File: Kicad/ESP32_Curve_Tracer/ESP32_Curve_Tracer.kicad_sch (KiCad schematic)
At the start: 69 parts, among them J1 PROBE_CH1-, J2 PROBE_CH2-, J3 PROBE_CH1_VIA1_16, J4 PROBE_CH2_VIA1_16, J5 PROBE_CH1+, J6 PROBE_CH2+, U1 DOIT-ESP32-DEVKIT-V1, U2 LMV324, U3 CD74HC4067M, U4 CD74HC4067M, U5 CD74HC4067M, U6 CD74HC4067M, U7 74HC595, U8 74HC595, U9 74HC595

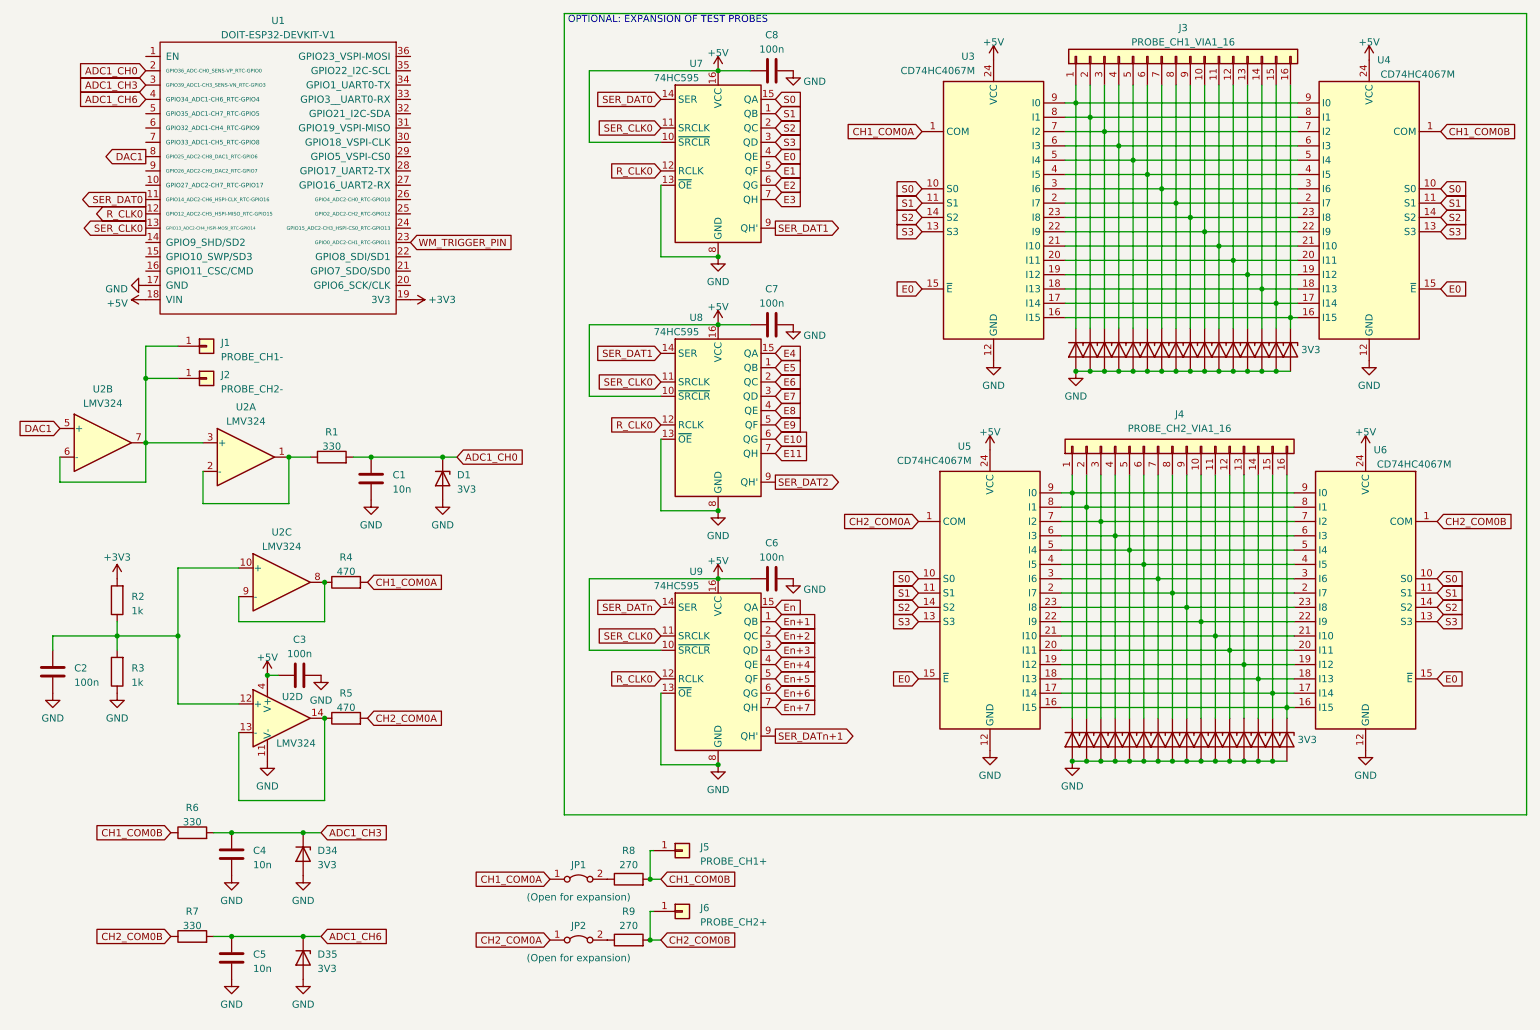
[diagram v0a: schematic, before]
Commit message: Update
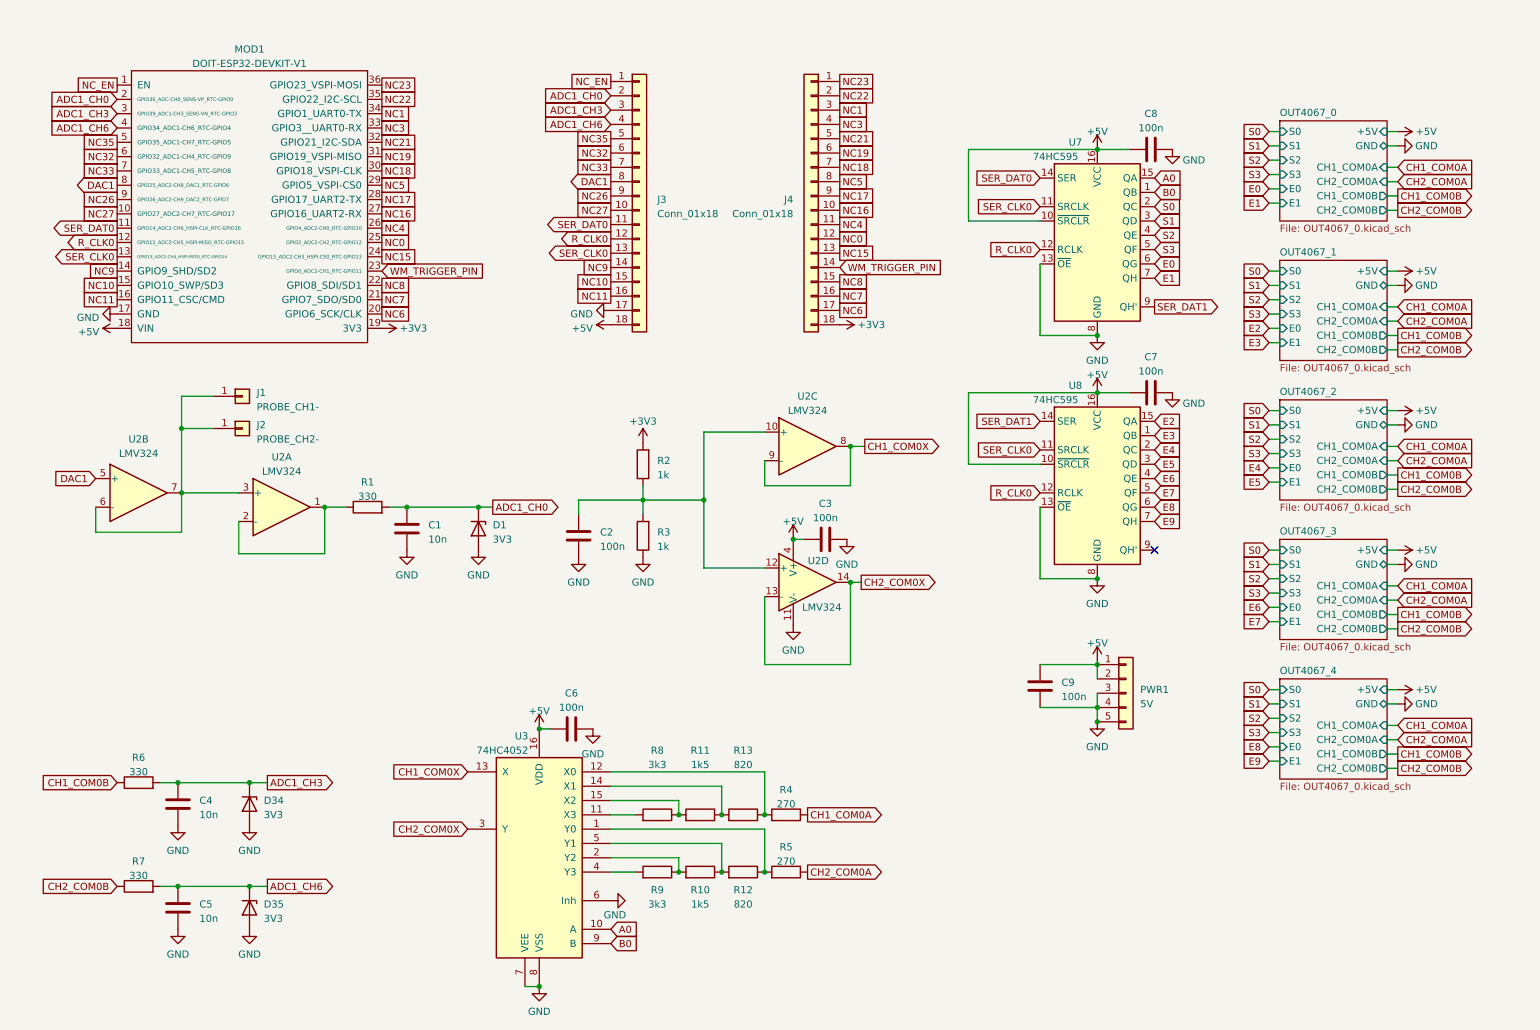
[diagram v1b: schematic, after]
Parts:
- removed D10, D11, D12, D13, D14, D15, D16, D17, D18, D19, D2, D20, D21, D22, D23, D24, D25, D26, D27, D28, D29, D3, D30, D31, D32, D33, D4, D5, D6, D7, D8, D9: 3V3, symbol Device:D_Zener
- removed J3: PROBE_CH1_VIA1_16, symbol Connector_Generic:Conn_01x16
- removed J4: PROBE_CH2_VIA1_16, symbol Connector_Generic:Conn_01x16
- removed J5: PROBE_CH1+, symbol Connector_Generic:Conn_01x01
- removed J6: PROBE_CH2+, symbol Connector_Generic:Conn_01x01
- removed JP1, JP2: (Open for expansion), symbol Jumper:Jumper_2_Bridged
- removed U3, U4, U5, U6: CD74HC4067M, Package_SO:SOIC-24W_7.5x15.4mm_P1.27mm, symbol 74xx:CD74HC4067M
- removed U9: 74HC595, symbol 74xx:74HC595
- added C9: 100n, Capacitor_SMD:C_0805_2012Metric_Pad1.18x1.45mm_HandSolder, symbol Device:C
- added J3, J4: Conn_01x18, Connector_PinSocket_2.54mm:PinSocket_1x18_P2.54mm_Vertical, symbol Connector_Generic:Conn_01x18
- added PWR1: 5V, Connector_PinHeader_2.54mm:PinHeader_1x05_P2.54mm_Vertical, symbol Connector_Generic:Conn_01x05
- added R10, R11: 1k5, Resistor_SMD:R_0805_2012Metric_Pad1.20x1.40mm_HandSolder, symbol Device:R
- added R12, R13: 820, Resistor_SMD:R_0805_2012Metric_Pad1.20x1.40mm_HandSolder, symbol Device:R
- added U3: 74HC4052, Package_SO:SOP-16_3.9x9.9mm_P1.27mm, symbol 4xxx:4052
- C1, C2, C3, C4, C5, C6, C7, C8: footprint (none) -> Capacitor_SMD:C_0805_2012Metric_Pad1.18x1.45mm_HandSolder
- D1, D34, D35: footprint (none) -> Diode_SMD:D_SOD-323_HandSoldering
- J1, J2: footprint (none) -> Connector_PinHeader_2.54mm:PinHeader_1x01_P2.54mm_Vertical
- MOD1: renamed from U1; footprint (none) -> ESP32:ESP32-DOIT-DEVKIT
- R1, R2, R3, R6, R7: footprint (none) -> Resistor_SMD:R_0805_2012Metric_Pad1.20x1.40mm_HandSolder
- R4, R5: value 470 -> 270; footprint (none) -> Resistor_SMD:R_0805_2012Metric_Pad1.20x1.40mm_HandSolder
- R8, R9: value 270 -> 3k3; footprint (none) -> Resistor_SMD:R_0805_2012Metric_Pad1.20x1.40mm_HandSolder
- U2: footprint (none) -> Package_SO:SO-14_3.9x8.65mm_P1.27mm
- U7, U8: footprint (none) -> Package_SO:SOP-16_3.9x9.9mm_P1.27mm
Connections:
- net E10 is gone; now on net E8: U8.6 (QG)
- net E11 is gone; now on net E9: U8.7 (QH)
- net +3V3: now also J4.18 (Pin_18)
- net +5V: now also C9.1, J3.18 (Pin_18), PWR1.1 (Pin_1), PWR1.2 (Pin_2), U3.16 (VDD)
- net ADC1_CH0: now also J3.2 (Pin_2)
- net ADC1_CH3: now also J3.3 (Pin_3)
- net ADC1_CH6: now also J3.4 (Pin_4)
- net CH1_COM0A: now also R4.1; no longer R4.2
- net CH1_COM0B: no longer R8.2
- net CH2_COM0A: now also R5.1; no longer R5.2
- net CH2_COM0B: no longer R9.2
- net DAC1: now also J3.8 (Pin_8)
- net E0: now also U7.6 (QG); no longer U7.4 (QE)
- net E1: now also U7.7 (QH); no longer U7.5 (QF)
- net E2: now also U8.15 (QA); no longer U7.6 (QG)
- net E3: now also U8.1 (QB); no longer U7.7 (QH)
- net E4: now also U8.2 (QC); no longer U8.15 (QA)
- net E5: now also U8.3 (QD); no longer U8.1 (QB)
- net E6: now also U8.4 (QE); no longer U8.2 (QC)
- net E7: now also U8.5 (QF); no longer U8.3 (QD)
- net E8: no longer U8.4 (QE)
- net E9: no longer U8.5 (QF)
- net GND: now also C9.2, J3.17 (Pin_17), PWR1.3 (Pin_3), PWR1.4 (Pin_4), PWR1.5 (Pin_5), U3.6 (Inh), U3.7 (VEE), U3.8 (VSS)
- net R_CLK0: now also J3.12 (Pin_12)
- net S0: now also U7.2 (QC); no longer U7.15 (QA)
- net S1: now also U7.3 (QD); no longer U7.1 (QB)
- net S2: now also U7.4 (QE); no longer U7.2 (QC)
- net S3: now also U7.5 (QF); no longer U7.3 (QD)
- net SER_CLK0: now also J3.13 (Pin_13)
- net SER_DAT0: now also J3.11 (Pin_11)
- net WM_TRIGGER_PIN: now also J4.14 (Pin_14)
- net at R9.1: now also R10.2, U3.2 (Y2)
- net at R8.1: now also R11.2, U3.15 (X2)
- net CH2_COM0X: now reaches U2.13 (-), U2.14
- net CH2_COM0X: now also U3.3 (Y); no longer R5.1
- net NC_EN: now reaches MOD1.1 (EN)
- net NC_EN: now also J3.1 (Pin_1)
- net NC27: now reaches MOD1.10 (GPIO27_ADC2-CH7_RTC-GPIO17)
- net NC27: now also J3.10 (Pin_10)
- net NC9: now reaches MOD1.14 (GPIO9_SHD/SD2)
- net NC9: now also J3.14 (Pin_14)
- net NC10: now reaches MOD1.15 (GPIO10_SWP/SD3)
- net NC10: now also J3.15 (Pin_15)
- net NC11: now reaches MOD1.16 (GPIO11_CSC/CMD)
- net NC11: now also J3.16 (Pin_16)
- net NC6: now reaches MOD1.20 (GPIO6_SCK/CLK)
- net NC6: now also J4.17 (Pin_17)
- net NC7: now reaches MOD1.21 (GPIO7_SDO/SD0)
- net NC7: now also J4.16 (Pin_16)
- net NC8: now reaches MOD1.22 (GPIO8_SDI/SD1)
- net NC8: now also J4.15 (Pin_15)
- net NC15: now reaches MOD1.24 (GPIO15_ADC2-CH3_HSPI-CS0_RTC-GPIO13)
- net NC15: now also J4.13 (Pin_13)
- net NC0: now reaches MOD1.25 (GPIO2_ADC2-CH2_RTC-GPIO12)
- net NC0: now also J4.12 (Pin_12)
- net NC4: now reaches MOD1.26 (GPIO4_ADC2-CH0_RTC-GPIO10)
- net NC4: now also J4.11 (Pin_11)
- net NC16: now reaches MOD1.27 (GPIO16_UART2-RX)
- net NC16: now also J4.10 (Pin_10)
- net NC17: now reaches MOD1.28 (GPIO17_UART2-TX)
- net NC17: now also J4.9 (Pin_9)
- net NC5: now reaches MOD1.29 (GPIO5_VSPI-CS0)
- net NC5: now also J4.8 (Pin_8)
- net NC18: now reaches MOD1.30 (GPIO18_VSPI-CLK)
- net NC18: now also J4.7 (Pin_7)
- net NC19: now reaches MOD1.31 (GPIO19_VSPI-MISO)
- net NC19: now also J4.6 (Pin_6)
- net NC21: now reaches MOD1.32 (GPIO21_I2C-SDA)
- net NC21: now also J4.5 (Pin_5)
- net NC3: now reaches MOD1.33 (GPIO3__UART0-RX)
- net NC3: now also J4.4 (Pin_4)
- net NC1: now reaches MOD1.34 (GPIO1_UART0-TX)
- net NC1: now also J4.3 (Pin_3)
- net NC22: now reaches MOD1.35 (GPIO22_I2C-SCL)
- net NC22: now also J4.2 (Pin_2)
- net NC23: now reaches MOD1.36 (GPIO23_VSPI-MOSI)
- net NC23: now also J4.1 (Pin_1)
- net NC35: now reaches MOD1.5 (GPIO35_ADC1-CH7_RTC-GPIO5)
- net NC35: now also J3.5 (Pin_5)
- net NC32: now reaches MOD1.6 (GPIO32_ADC1-CH4_RTC-GPIO9)
- net NC32: now also J3.6 (Pin_6)
- net NC33: now reaches MOD1.7 (GPIO33_ADC1-CH5_RTC-GPIO8)
- net NC33: now also J3.7 (Pin_7)
- net NC26: now reaches MOD1.9 (GPIO26_ADC2-CH9_DAC2_RTC-GPIO7)
- net NC26: now also J3.9 (Pin_9)
- net CH1_COM0X: now reaches U2.8, U2.9 (-)
- net CH1_COM0X: now also U3.13 (X); no longer R4.1
- net SER_DAT2: no longer names the net of U8.9 (QH')
- new net: R11.1, R13.2, U3.14 (X1)
- new net: R13.1, R4.2, U3.12 (X0)
- new net: R12.1, R5.2, U3.1 (Y0)
- new net: R10.1, R12.2, U3.5 (Y1)
- new net: R9.2, U3.4 (Y3)
- new net: R8.2, U3.11 (X3)
- new net A0: U3.10 (A), U7.15 (QA)
- new net B0: U3.9 (B), U7.1 (QB)
- no-connect marks 0 -> 1
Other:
- added sheet OUT4067_0 (OUT4067_0.kicad_sch)
- added sheet OUT4067_1 (OUT4067_0.kicad_sch)
- added sheet OUT4067_2 (OUT4067_0.kicad_sch)
- added sheet OUT4067_3 (OUT4067_0.kicad_sch)
- added sheet OUT4067_4 (OUT4067_0.kicad_sch)
- note removed: "OPTIONAL: EXPANSION OF TEST PROBES"
- moved on the sheet: C1, C2, C3, C4, C5, C7, C8, D1, D34, D35, J1, J2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
